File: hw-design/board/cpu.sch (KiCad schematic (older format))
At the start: 23 parts, among them P1 CHAIN, P2 USB_OTG, P3 SWD, Q7 BC857, SW1 SW_PUSH, U4 LPC11U24FBD48/401, Y1 12MHz

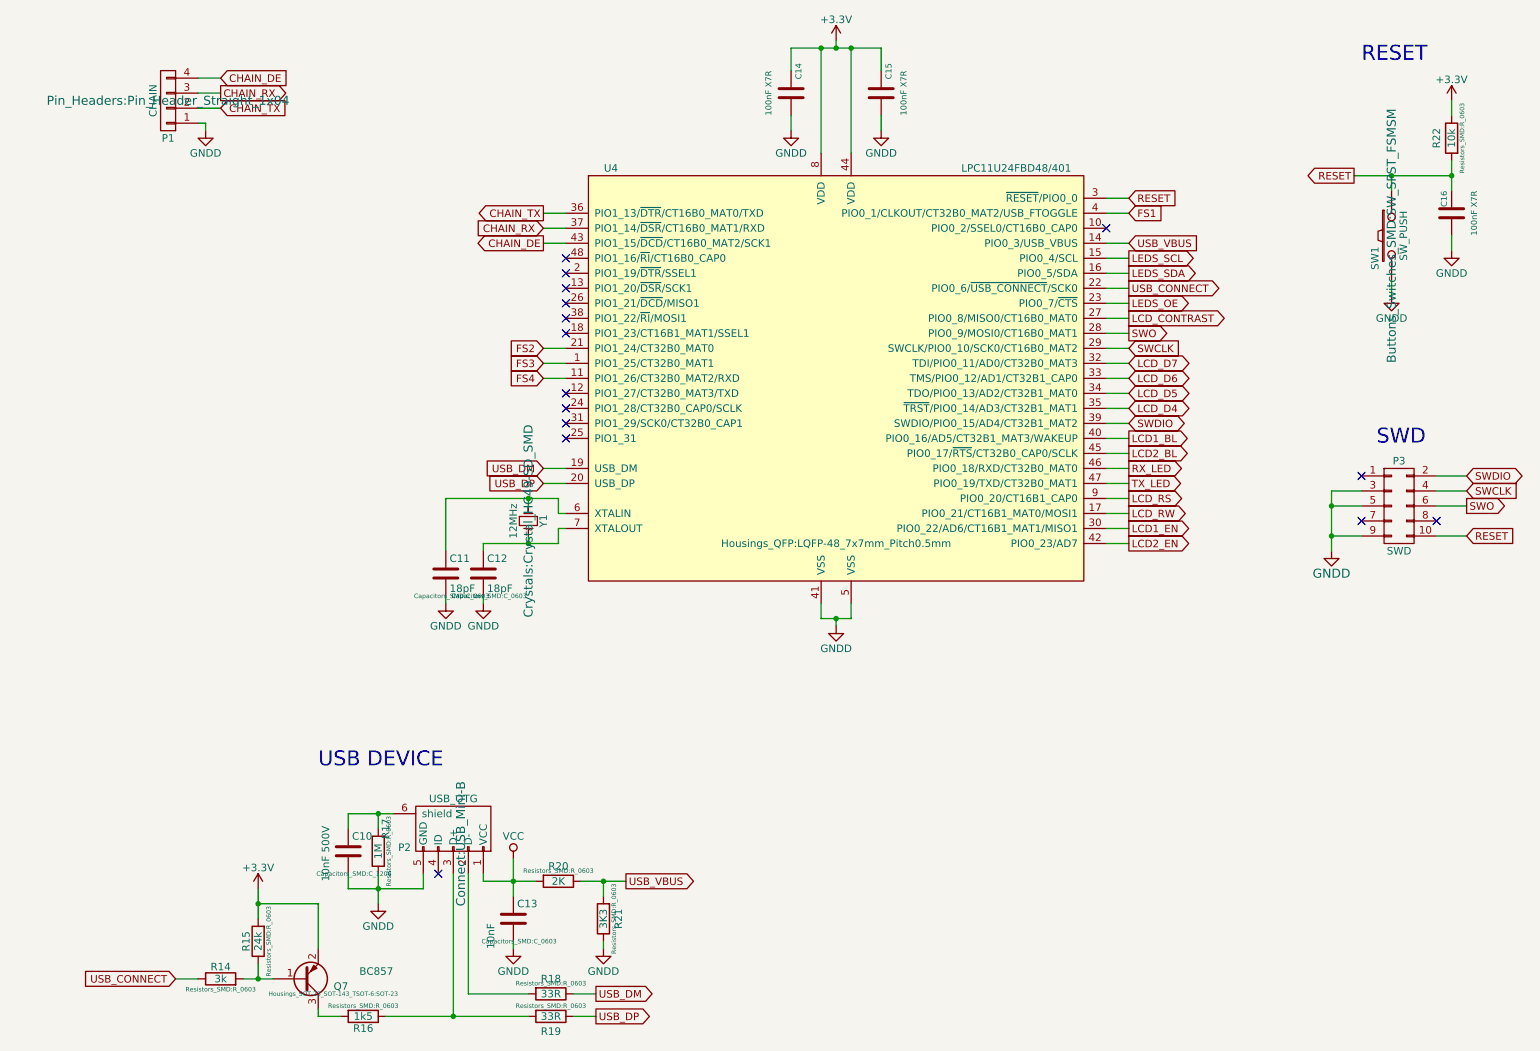
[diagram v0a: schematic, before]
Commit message: sch: schematic files reorganized, new sheets for usb and rear board
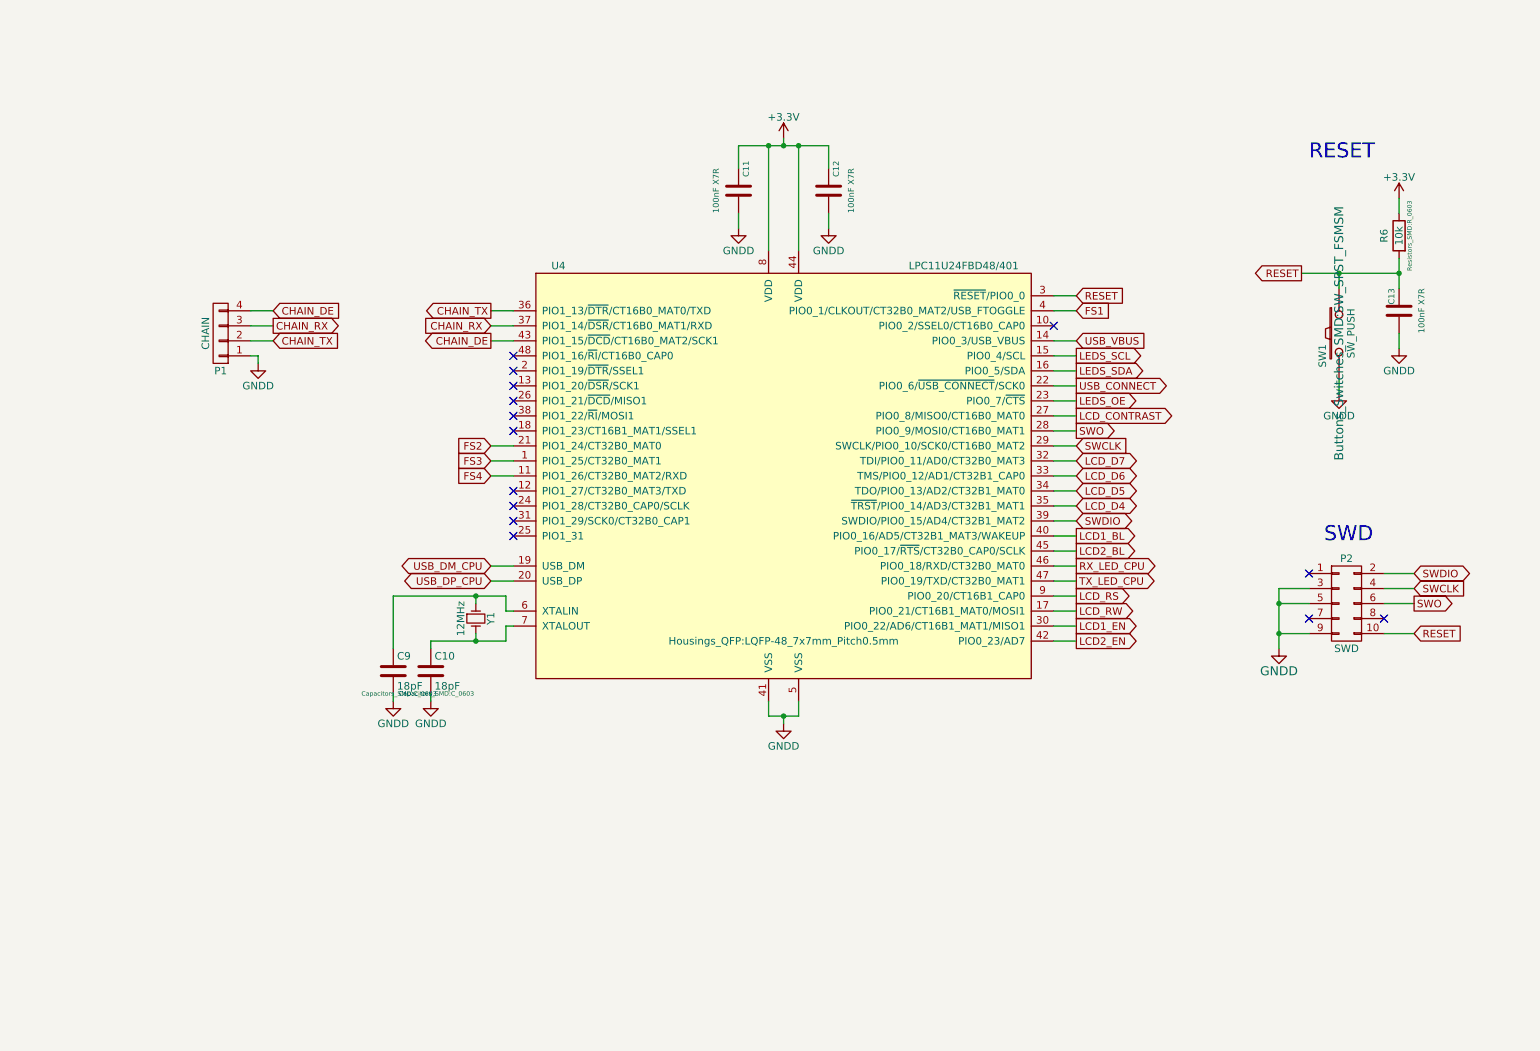
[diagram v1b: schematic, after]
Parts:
- removed C10: 10nF 500V, Capacitors_SMD:C_1206, symbol C
- removed C13: 10nF, Capacitors_SMD:C_0603, symbol C
- removed P2: USB_OTG, Connect:USB_Mini-B, symbol USB_OTG
- removed Q7: BC857, Housings_SOT-23_SOT-143_TSOT-6:SOT-23, symbol Q_PNP_BEC
- removed R14: 3k, Resistors_SMD:R_0603, symbol R
- removed R15: 24k, Resistors_SMD:R_0603, symbol R
- removed R16: 1k5, Resistors_SMD:R_0603, symbol R
- removed R17: 1M, Resistors_SMD:R_0603, symbol R
- removed R18, R19: 33R, Resistors_SMD:R_0603, symbol R
- removed R20: 2K, Resistors_SMD:R_0603, symbol R
- removed R21: 3K3, Resistors_SMD:R_0603, symbol R
- renumbered C12 to C10, C14 to C11, C15 to C12, C16 to C13, C11 to C9, P3 to P2, R22 to R6
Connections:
- net RX_LED renamed RX_LED_CPU
- net TX_LED renamed TX_LED_CPU
- net USB_DM renamed USB_DM_CPU
- net USB_DP renamed USB_DP_CPU
- no-connect marks 15 -> 14
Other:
- note removed: "USB DEVICE"
- moved on the sheet: C10, C11, C12, C13, C9, P1, P2, R6, SW1, U4, Y1

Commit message: connecting foot leds directly to cpu
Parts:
- P1: footprint Pin_Headers:Pin_Header_Straight_1x04 -> Pin_Headers:Pin_Header_Straight_1x03; symbol CONN_01X04 -> CONN_01X03
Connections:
- net LEDS_SCL is gone; now on net FS3: U4.15 (PIO0_4/SCL)
- net LEDS_SDA is gone; now on net FS4: U4.16 (PIO0_5/SDA)
- net CHAIN_DE: no longer P1.4 (P4)
- net FS2: now also U4.10 (PIO0_2/SSEL0/CT16B0_CAP0); no longer U4.21 (PIO1_24/CT32B0_MAT0)
- net FS3: no longer U4.1 (PIO1_25/CT32B0_MAT1)
- net FS4: no longer U4.11 (PIO1_26/CT32B0_MAT2/RXD)
- net LED_B4: now reaches U4.12 (PIO1_27/CT32B0_MAT3/TXD)
- net LED_G1: now reaches U4.13 (PIO1_20/~DSR~/SCK1)
- net LED_G2: now reaches U4.18 (PIO1_23/CT16B1_MAT1/SSEL1)
- net LED_R1: now reaches U4.2 (PIO1_19/~DTR~/SSEL1)
- net LED_R4: now reaches U4.24 (PIO1_28/CT32B0_CAP0/SCLK)
- net LED_B2: now reaches U4.26 (PIO1_21/~DCD~/MISO1)
- net LED_G4: now reaches U4.31 (PIO1_29/SCK0/CT32B0_CAP1)
- net LED_R2: now reaches U4.38 (PIO1_22/~RI~/MOSI1)
- net LED_B1: now reaches U4.48 (PIO1_16/~RI~/CT16B0_CAP0)
- net LEDS_OE: no longer names the net of U4.23 (PIO0_7/~CTS~)
- net RX_LED_CPU: no longer names the net of U4.46 (PIO0_18/RXD/CT32B0_MAT0)
- net TX_LED_CPU: no longer names the net of U4.47 (PIO0_19/TXD/CT32B0_MAT1)
- new net LED_B3: U4.21 (PIO1_24/CT32B0_MAT0)
- new net LED_G3: U4.11 (PIO1_26/CT32B0_MAT2/RXD)
- new net LED_R3: U4.1 (PIO1_25/CT32B0_MAT1)
- no-connect marks 14 -> 7
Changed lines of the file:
@@
-$EndComp
-$Comp
-L LPC11U24FBD48/401 U4
-U 1 1 556F3A3A
-P 5550 3750
-F 0 "U4" H 4050 5150 50  0000 C CNN
-F 1 "LPC11U24FBD48/401" H 6750 5150 50  0000 C CNN
-F 2 "Housings_QFP:LQFP-48_7x7mm_Pitch0.5mm" H 5550 2650 50  0000 C CNN
-F 3 "" H 5500 3700 60  0000 C CNN
-F 4 "LPC11U24FBD48/401" H -350 650 50  0001 C CNN "MPN"
-	1    5550 3750
-	1    0    0    -1
 $EndComp
 $Comp
@@
 F 0 "C10" H 3225 5150 50  0000 L CNN
 F 1 "18pF" H 3225 4950 50  0000 L CNN
-F 2 "Capacitors_SMD:C_0603" H 3238 4900 30  0000 C CNN
+F 2 "Capacitors_SMD:C_0603" H 3238 4900 30  0001 C CNN
 F 3 "" H 3200 5050 60  0000 C CNN
 F 4 "C1608C0G1H180J080AA" H -350 650 50  0001 C CNN "MPN"
@@
 F 0 "C9" H 2975 5150 50  0000 L CNN
 F 1 "18pF" H 2975 4950 50  0000 L CNN
-F 2 "Capacitors_SMD:C_0603" H 2988 4900 30  0000 C CNN
+F 2 "Capacitors_SMD:C_0603" H 2988 4900 30  0001 C CNN
 F 3 "" H 2950 5050 60  0000 C CNN
 F 4 "C1608C0G1H180J080AA" H -350 650 50  0001 C CNN "MPN"
@@
 $EndComp
 $Comp
-L CONN_01X04 P1
+L CONN_01X03 P1
 U 1 1 557F309A
-P 1800 2800
-F 0 "P1" H 1800 3050 50  0000 C CNN
-F 1 "CHAIN" V 1900 2800 50  0000 C CNN
-F 2 "Pin_Headers:Pin_Header_Straight_1x04" H 1800 2800 60  0001 C CNN
-F 3 "" H 1800 2800 60  0000 C CNN
-F 4 "-" H 350 1550 50  0001 C CNN "MPN"
-	1    1800 2800
+P 1800 2850
+F 0 "P1" H 1800 3100 50  0000 C CNN
+F 1 "CHAIN" V 1900 2850 50  0000 C CNN
+F 2 "Pin_Headers:Pin_Header_Straight_1x03" H 1800 2850 60  0001 C CNN
+F 3 "" H 1800 2850 60  0000 C CNN
+F 4 "-" H 350 1600 50  0001 C CNN "MPN"
+	1    1800 2850
 	-1   0    0    1
 $EndComp
@@
 F 0 "R6" V 9750 2150 50  0000 C CNN
 F 1 "10k" V 9650 2150 50  0000 C CNN
-F 2 "Resistors_SMD:R_0603" V 9580 2150 30  0000 C CNN
+F 2 "Resistors_SMD:R_0603" V 9580 2150 30  0001 C CNN
 F 3 "" H 9650 2150 30  0000 C CNN
 F 4 "RMCF0603JT10K0" H -350 650 50  0001 C CNN "MPN"
@@
 F 0 "SW1" H 9400 2910 50  0000 C CNN
 F 1 "SW_PUSH" H 9250 2720 50  0000 C CNN
-F 2 "Buttons_Switches_SMD:SW_SPST_FSMSM" H 9250 2800 60  0000 C CNN
+F 2 "Buttons_Switches_SMD:SW_SPST_FSMSM" H 9250 2800 60  0001 C CNN
 F 3 "" H 9250 2800 60  0000 C CNN
 F 4 "FSMSM" H -350 650 50  0001 C CNN "MPN"
@@
 Text GLabel 2150 2750 2    50   Output ~ 0
 CHAIN_RX
-Text GLabel 2150 2650 2    50   Input ~ 0
-CHAIN_DE
 Text GLabel 9750 4600 2    50   Output ~ 0
 SWO
@@
 Text GLabel 7500 2650 2    50   Input ~ 0
 FS1
-Text GLabel 7500 4350 2    50   Output ~ 0
-RX_LED_CPU
-Text GLabel 7500 4450 2    50   Output ~ 0
-TX_LED_CPU
-Text GLabel 7500 3050 2    50   Output ~ 0
-LEDS_SDA
-Text GLabel 7500 2950 2    50   Output ~ 0
-LEDS_SCL
-Text GLabel 7500 3250 2    50   Output ~ 0
-LEDS_OE
-Text GLabel 3600 3550 0    50   Input ~ 0
+Text GLabel 7500 2750 2    50   Input ~ 0
 FS2
-Text GLabel 3600 3650 0    50   Input ~ 0
+Text GLabel 7500 2950 2    50   Input ~ 0
 FS3
-Text GLabel 3600 3750 0    50   Input ~ 0
+Text GLabel 7500 3050 2    50   Input ~ 0
 FS4
 Text GLabel 7500 3650 2    50   BiDi ~ 0
@@
 	2150 2750 2000 2750
 Wire Wire Line
-	2000 2650 2150 2650
-Wire Wire Line
 	2000 2950 2050 2950
 Wire Wire Line
@@
 	7350 2650 7500 2650
 Wire Wire Line
-	7500 4350 7350 4350
-Wire Wire Line
-	7500 4450 7350 4450
-Wire Wire Line
-	7350 2950 7500 2950
+	7500 2750 7350 2750
+Wire Wire Line
+	7500 2950 7350 2950
 Wire Wire Line
 	7500 3050 7350 3050
-Wire Wire Line
-	7500 3250 7350 3250
-Wire Wire Line
-	3750 3550 3600 3550
-Wire Wire Line
-	3750 3650 3600 3650
-Wire Wire Line
-	3750 3750 3600 3750
 Wire Wire Line
 	7500 3650 7350 3650
@@
 NoConn ~ 9050 4400
 NoConn ~ 9550 4700
-NoConn ~ 3750 3350
-NoConn ~ 3750 3850
-NoConn ~ 7350 2750
-NoConn ~ 3750 2950
-NoConn ~ 3750 3950
-NoConn ~ 3750 4050
 NoConn ~ 3750 4150
-NoConn ~ 3750 3450
-NoConn ~ 3750 3050
-NoConn ~ 3750 3150
-NoConn ~ 3750 3250
+Text GLabel 3600 3050 0    50   Output ~ 0
+LED_R1
+Text GLabel 3600 3150 0    50   Output ~ 0
+LED_G1
+Text GLabel 3600 2950 0    50   Output ~ 0
+LED_B1
+Text GLabel 3600 3350 0    50   Output ~ 0
+LED_R2
+Text GLabel 3600 3450 0    50   Output ~ 0
+LED_G2
+Text GLabel 3600 3250 0    50   Output ~ 0
+LED_B2
+Text GLabel 3600 3650 0    50   Output ~ 0
+LED_R3
+Text GLabel 3600 3750 0    50   Output ~ 0
+LED_G3
+Text GLabel 3600 3550 0    50   Output ~ 0
+LED_B3
+Text GLabel 3600 3950 0    50   Output ~ 0
+LED_R4
+Text GLabel 3600 4050 0    50   Output ~ 0
+LED_G4
+Text GLabel 3600 3850 0    50   Output ~ 0
+LED_B4
+$Comp
+L LPC11U24FBD48/401 U4
+U 1 1 556F3A3A
+P 5550 3750
+F 0 "U4" H 4050 5150 50  0000 C CNN
+F 1 "LPC11U24FBD48/401" H 6750 5150 50  0000 C CNN
+F 2 "Housings_QFP:LQFP-48_7x7mm_Pitch0.5mm" H 5550 2650 50  0000 C CNN
+F 3 "" H 5500 3700 60  0000 C CNN
+F 4 "LPC11U24FBD48/401" H -350 650 50  0001 C CNN "MPN"
+	1    5550 3750
+	1    0    0    -1
+$EndComp
+Wire Wire Line
+	3600 2950 3750 2950
+Wire Wire Line
+	3600 3050 3750 3050
+Wire Wire Line
+	3750 3150 3600 3150
+Wire Wire Line
+	3600 3250 3750 3250
+Wire Wire Line
+	3600 3350 3750 3350
+Wire Wire Line
+	3750 3450 3600 3450
+Wire Wire Line
+	3600 3550 3750 3550
+Wire Wire Line
+	3750 3650 3600 3650
+Wire Wire Line
+	3600 3750 3750 3750
+Wire Wire Line
+	3750 3850 3600 3850
+Wire Wire Line
+	3600 3950 3750 3950
+Wire Wire Line
+	3750 4050 3600 4050
+NoConn ~ 7350 4350
+NoConn ~ 7350 4450
+NoConn ~ 7350 3250
 $EndSCHEMATC
